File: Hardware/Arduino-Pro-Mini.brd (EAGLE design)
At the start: 17.8 x 33 mm, 26 parts, among them Q1 8/16MHz, U1 ATMEGA328, U2 MIC5205

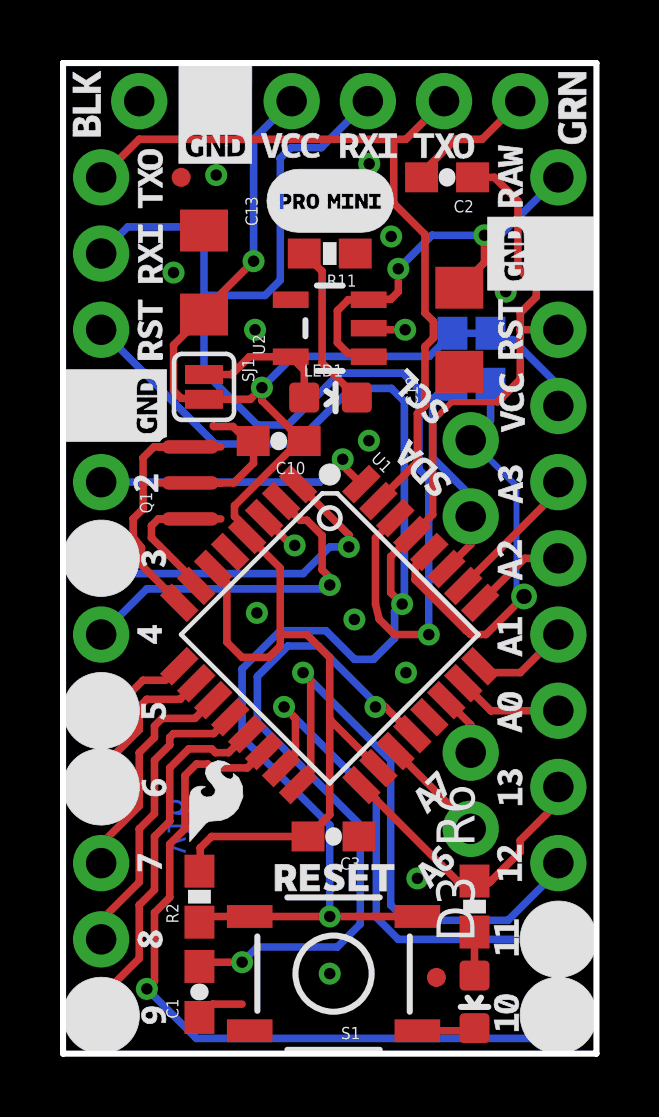
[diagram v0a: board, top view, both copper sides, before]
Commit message: Incremented version numbers
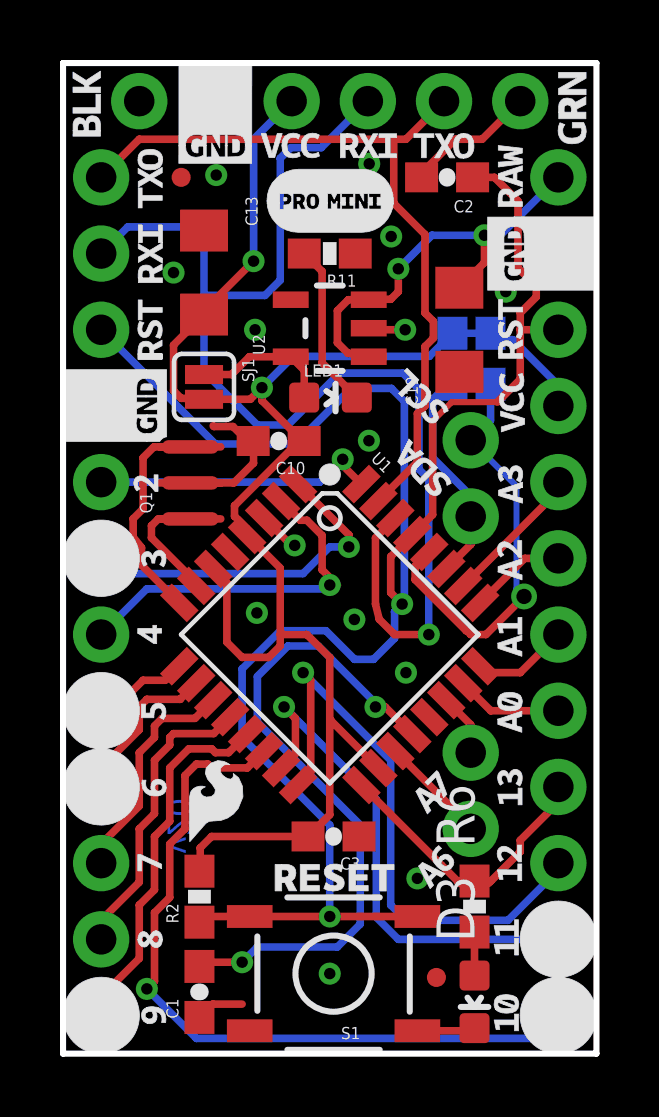
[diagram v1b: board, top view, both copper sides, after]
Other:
- board text added: "v20"
- board text removed: "v16"
